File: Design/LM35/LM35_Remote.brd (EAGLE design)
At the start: 16.2 x 52.1 mm, 6 parts

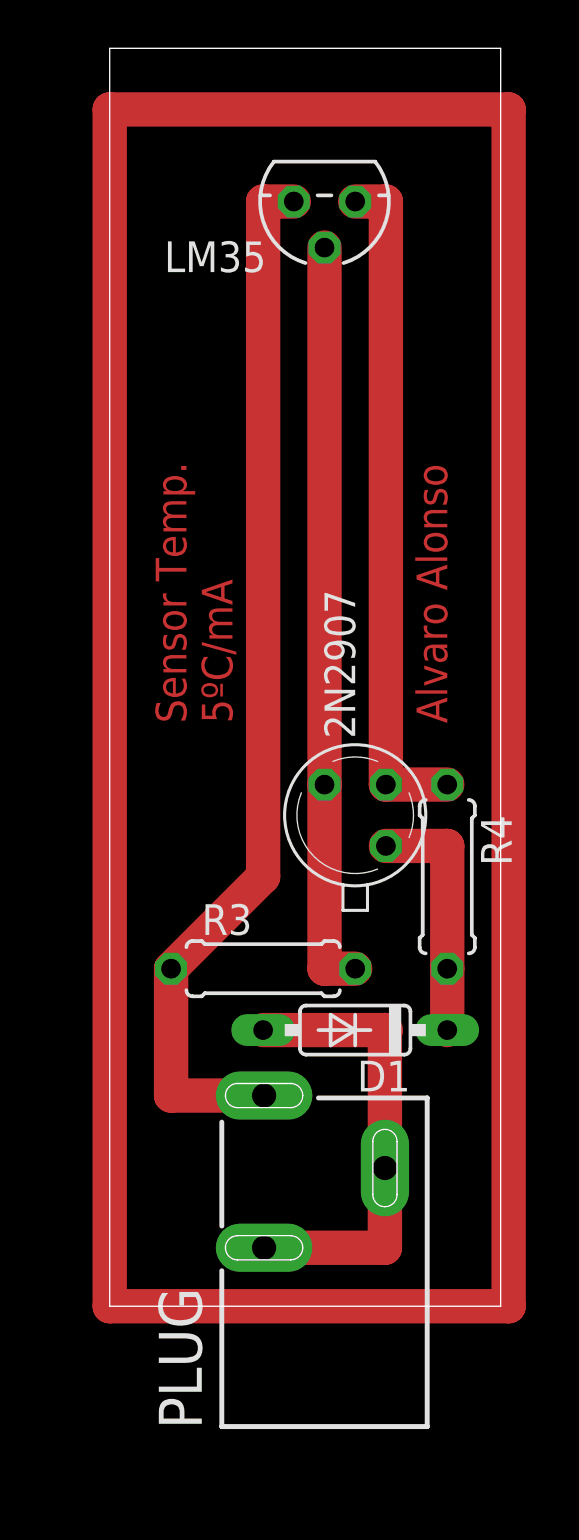
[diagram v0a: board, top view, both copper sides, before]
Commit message: Fix Doc files
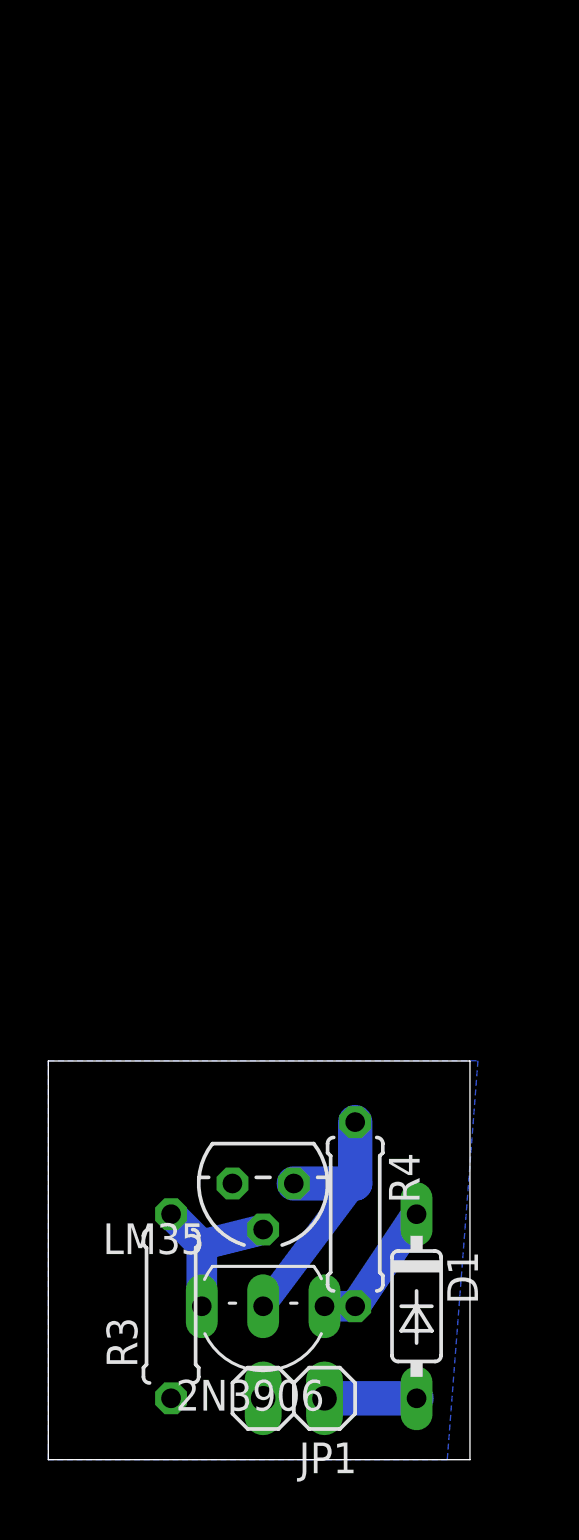
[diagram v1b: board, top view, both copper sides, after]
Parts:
- removed 2N2907: (no value), transistor:TO18
- removed PLUG: (no value), con-shiua-chyuan:SCD-014-A
- added 2N3906: (no value), transistor-neu-to92:TO92-EBC
- added JP1: (no value), pinhead:1X02
- moved LM35 40.7 mm to (8.89, 11.4)
- moved R3 14.5 mm to (5.08, 6.35), turned to 90 degrees
- moved R4 14.5 mm to (12.7, 10.2)
- moved D1 11.7 mm to (15.2, 6.35), turned to 270 degrees
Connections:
- removed net N$4: LM35.3, PLUG.1, R3.1
- removed net N$7: D1.A, PLUG.2, PLUG.3
- new net IN: D1.A, JP1.1
- new net OUT: JP1.2, LM35.3, R3.1
- net N$1: now also 2N3906.B; no longer 2N2907.2
- net N$2: now also 2N3906.C; no longer 2N2907.3
- net N$3: now also 2N3906.E; no longer 2N2907.1
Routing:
- net N$6: track 132.1 -> 0.00 mm
- net N$4: track 43.7 -> 0.00 mm
- net N$2: track 31.1 -> 6.95 mm
- net N$7: track 19.1 -> 0.00 mm
- net N$1: track 27.9 -> 11.4 mm
- net N$3: track 10.2 -> 5.85 mm
- net IN: track 0.00 -> 3.81 mm
- added copper zone on layer 16, net OUT
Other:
- board size 16.2 x 52.1 mm -> 17.4 x 16.5 mm
- board text removed: "Alvaro Alonso"
- board text removed: "Sensor Temp. 5ºC/mA"
